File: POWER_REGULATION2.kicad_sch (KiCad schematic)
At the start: 72 parts, among them Q8 FDV301N, U19 NL17SZ17XV5T2G, U20 FPF1018, U21 NC7WZ07P6X, U22 TPS65400RGZT, U9 SIP32510DT-T1-GE3

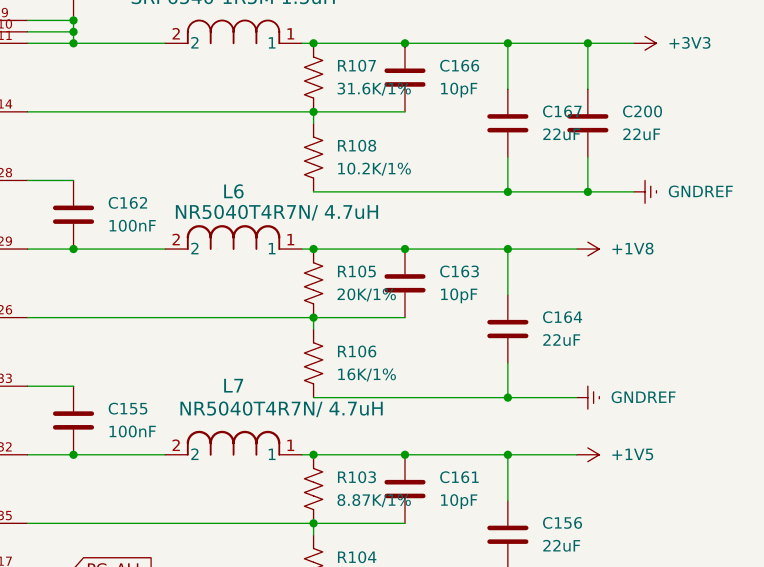
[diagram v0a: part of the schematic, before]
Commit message: update
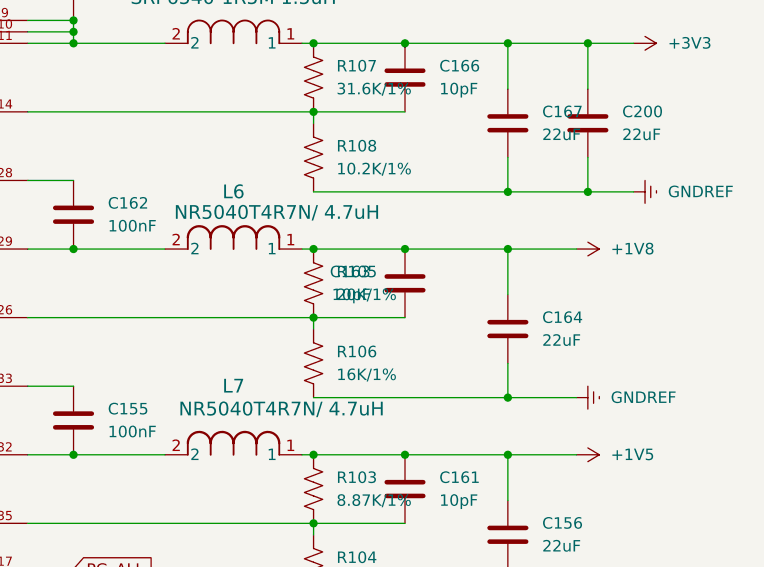
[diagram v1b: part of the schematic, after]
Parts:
- C155, C162, C165, C168: footprint footprints:C_0402 -> footprints:C_0201_0603Metric
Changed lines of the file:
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@@
 			)
 		)
-		(property "Footprint" "footprints:C_0402"
+		(property "Footprint" "footprints:C_0201_0603Metric"
 			(at 192.7352 110.49 0)
 			(effects
@@
 			)
 		)
-		(property "Footprint" "footprints:C_0402"
+		(property "Footprint" "footprints:C_0201_0603Metric"
 			(at 192.7352 62.23 0)
 			(effects
@@
 			)
 		)
-		(property "Footprint" "footprints:C_0402"
+		(property "Footprint" "footprints:C_0201_0603Metric"
 			(at 192.7352 87.63 0)
 			(effects
@@
 		(lib_id "Device:C")
 		(at 228.6 91.44 0)
+		(mirror y)
 		(unit 1)
 		(exclude_from_sim no)
@@
 		(on_board yes)
 		(dnp no)
-		(fields_autoplaced yes)
 		(property "Reference" "C163"
-			(at 232.41 90.1699 0)
+			(at 224.79 90.1699 0)
 			(effects
 				(font
@@
 		)
 		(property "Value" "10pF"
-			(at 232.41 92.7099 0)
+			(at 224.79 92.7099 0)
 			(effects
 				(font
@@
 		)
 		(property "Footprint" "footprints:C_0201_0603Metric"
-			(at 229.5652 95.25 0)
+			(at 227.6348 95.25 0)
 			(effects
 				(font
@@
 			)
 		)
-		(property "Footprint" "footprints:C_0402"
+		(property "Footprint" "footprints:C_0201_0603Metric"
 			(at 192.7352 35.56 0)
 			(effects

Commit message: update
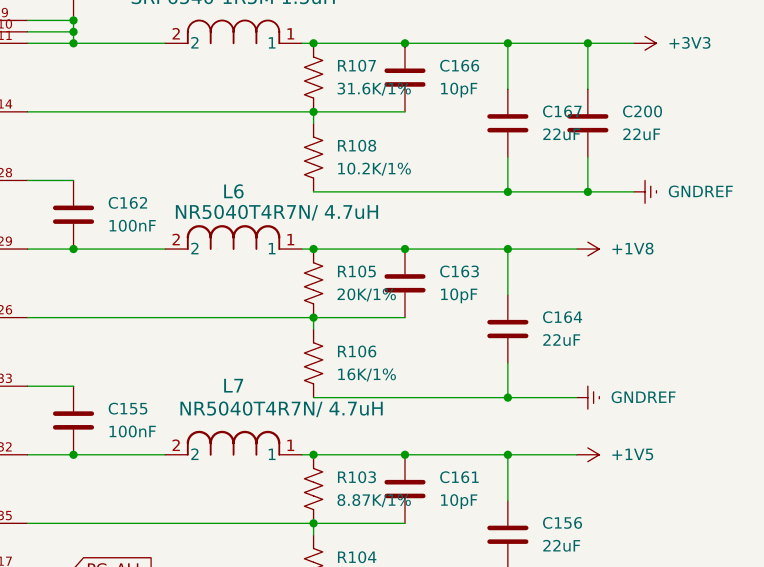
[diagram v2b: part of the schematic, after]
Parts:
- C155, C162, C165, C168: footprint footprints:C_0201_0603Metric -> footprints:C_0402
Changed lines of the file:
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@@
 			)
 		)
-		(property "Footprint" "footprints:C_0201_0603Metric"
+		(property "Footprint" "footprints:C_0402"
 			(at 192.7352 110.49 0)
 			(effects
@@
 			)
 		)
-		(property "Footprint" "footprints:C_0201_0603Metric"
+		(property "Footprint" "footprints:C_0402"
 			(at 192.7352 62.23 0)
 			(effects
@@
 			)
 		)
-		(property "Footprint" "footprints:C_0201_0603Metric"
+		(property "Footprint" "footprints:C_0402"
 			(at 192.7352 87.63 0)
 			(effects
@@
 		(lib_id "Device:C")
 		(at 228.6 91.44 0)
-		(mirror y)
 		(unit 1)
 		(exclude_from_sim no)
@@
 		(on_board yes)
 		(dnp no)
+		(fields_autoplaced yes)
 		(property "Reference" "C163"
-			(at 224.79 90.1699 0)
+			(at 232.41 90.1699 0)
 			(effects
 				(font
@@
 		)
 		(property "Value" "10pF"
-			(at 224.79 92.7099 0)
+			(at 232.41 92.7099 0)
 			(effects
 				(font
@@
 		)
 		(property "Footprint" "footprints:C_0201_0603Metric"
-			(at 227.6348 95.25 0)
+			(at 229.5652 95.25 0)
 			(effects
 				(font
@@
 			)
 		)
-		(property "Footprint" "footprints:C_0201_0603Metric"
+		(property "Footprint" "footprints:C_0402"
 			(at 192.7352 35.56 0)
 			(effects
